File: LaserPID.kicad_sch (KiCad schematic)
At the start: 59 parts, among them P1 POWER, P2 IN1, P3 IN2, P4 Out, P5 RST, SW1 SW_DPDT_x2, U1 INA105, U2 LM741, U3 LM741, U4 LM741, U6 LM741, U7 DG419

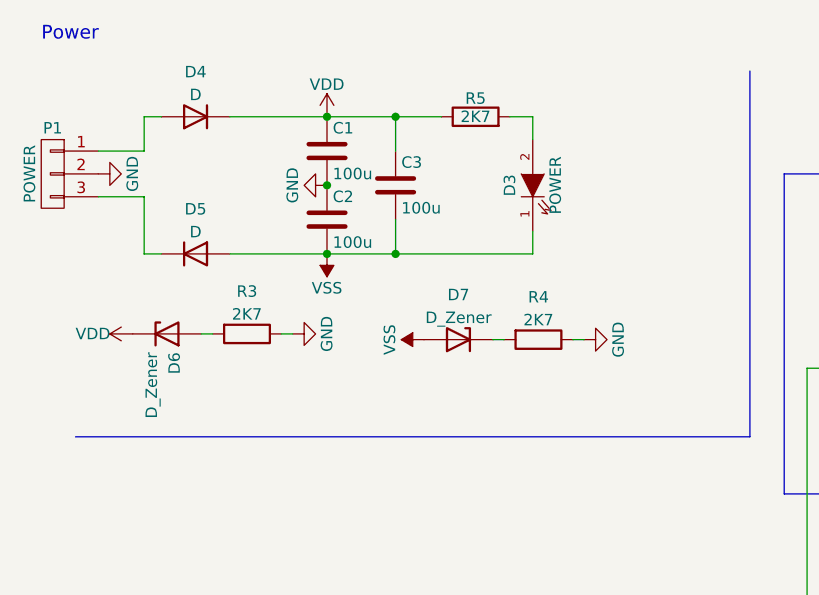
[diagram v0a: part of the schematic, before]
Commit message: Updated board, sent for production
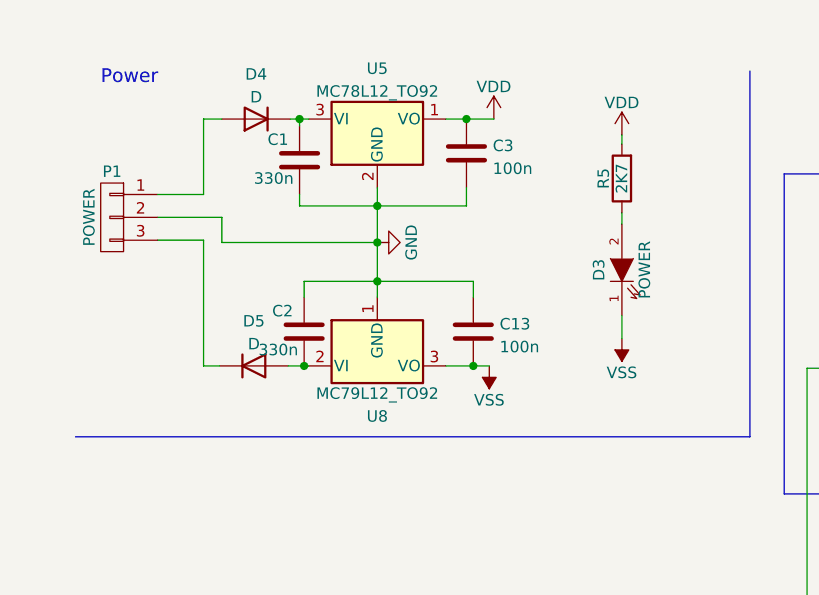
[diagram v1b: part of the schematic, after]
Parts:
- removed D6, D7: D_Zener, pi-servo-board:DIODE-SOD-123, symbol Device:D_Zener
- removed R3, R4: 2K7, Resistor_SMD:R_1206_3216Metric_Pad1.30x1.75mm_HandSolder, symbol Device:R
- added C13: 100n, Capacitor_SMD:C_1206_3216Metric_Pad1.33x1.80mm_HandSolder, symbol Device:C
- added U5: MC78L12_TO92, Package_TO_SOT_THT:TO-92_Inline, symbol Regulator_Linear:MC78L12_TO92
- added U8: MC79L12_TO92, Package_TO_SOT_THT:TO-92_Inline, symbol pi-servo-board:MC79L12_TO92
- C1, C2: value 100u -> 330n; footprint Capacitor_THT:CP_Radial_D10.0mm_P5.00mm -> Capacitor_SMD:C_1206_3216Metric_Pad1.33x1.80mm_HandSolder; Digikey Part Number 493-17046-ND -> 4713-GMC31X7R334K50NTCT-ND
- C3: value 100u -> 100n; footprint Capacitor_THT:CP_Radial_D10.0mm_P5.00mm -> Capacitor_SMD:C_1206_3216Metric_Pad1.33x1.80mm_HandSolder; Digikey Part Number 493-17046-ND -> 478-1556-1-ND
- U2, U3, U4, U6: Digikey Part Number OP07DNZ-ND -> 296-34251-5-ND
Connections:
- net GND: now also C3.2, C13.1, U5.2 (GND), U8.1 (GND)
- net VDD: now also R5.2, U5.1 (VO); no longer C1.1, D4.1 (K), R5.1
- net VSS: now also C13.2, U8.3 (VO); no longer C2.2, C3.2, D5.2 (A)
- net at D3.2 (A): now also R5.1; no longer R5.2
- new net: C2.2, D5.2 (A), U8.2 (VI)
- new net: C1.1, D4.1 (K), U5.3 (VI)
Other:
- moved on the sheet: D3, D4, D5, P1, R5
